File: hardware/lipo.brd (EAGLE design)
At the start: 33.5 x 34.6 mm, 57 parts, among them J1 MICRO_USB_B_HIROSE_ZX62-B-5PA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, Q1 IRLML6402, SW1 TVAF06-A020B-R, U1 LT6106CS5#PBF, U2 NJM12888F, U3 MCP73831, U5 TCK106AF,LF, X1 FA-238

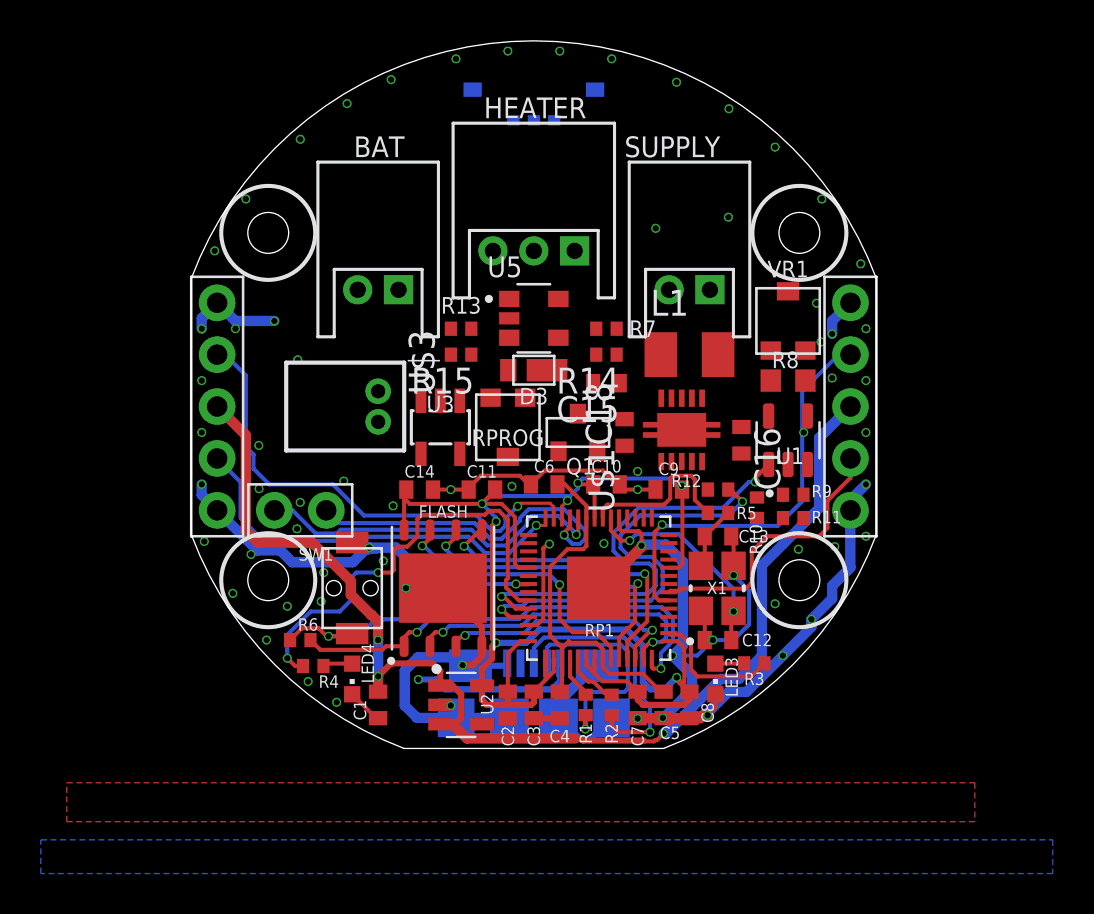
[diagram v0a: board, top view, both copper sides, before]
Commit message: アナログ入力を修正
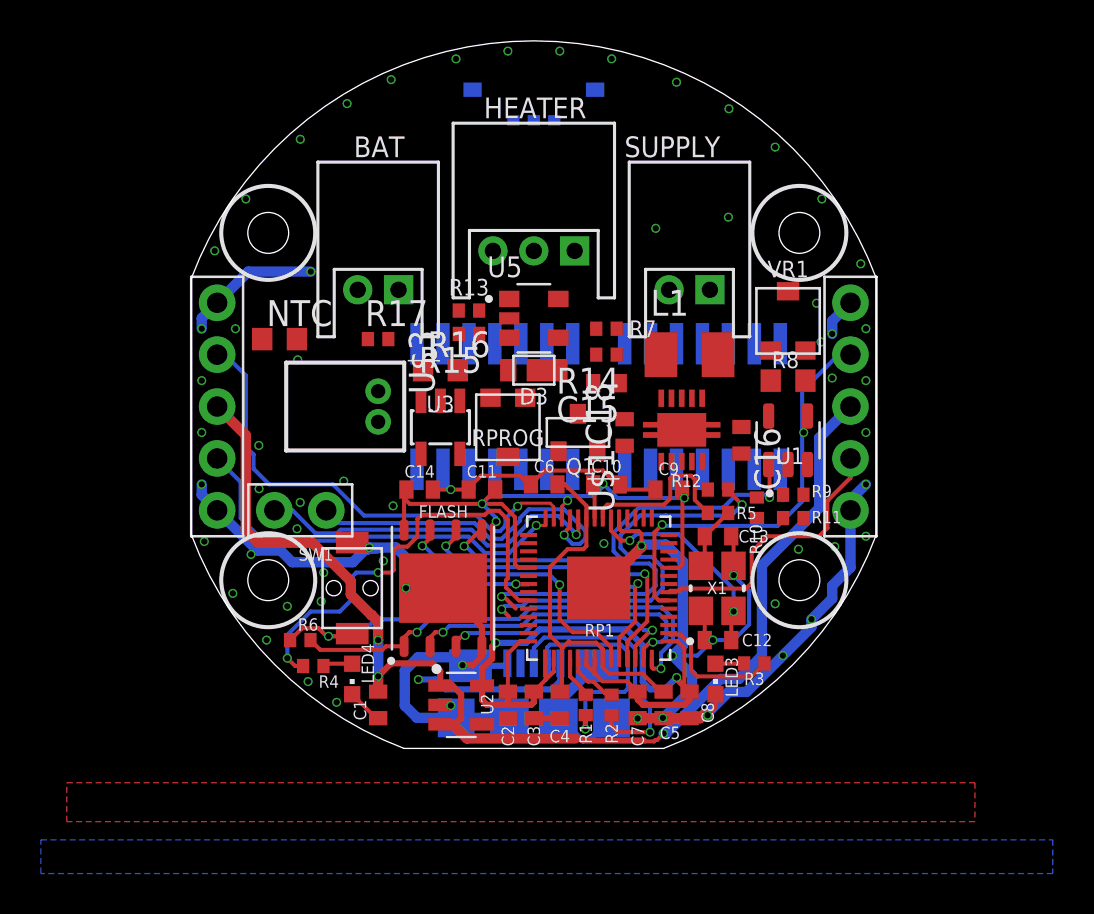
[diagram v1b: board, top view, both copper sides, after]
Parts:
- added IC1, IC2: 4066D, 40xx:SO14
- added NTC: 10k, rcl:R0603
- added R16: 0.033, rcl:R0603
- added R17: 10k, rcl:R0402
- moved R15 1.09 mm to (-3.17, 3.56)
- moved R13 0.97 mm to (-3.17, 4.70)
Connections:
- removed net ADC3: RP1.41
- removed net I2C0_SDA: RP1.11
- removed net I2C1_SCL: RP1.9
- removed net I2C1_SDA: RP1.8
- removed net I2C_SCL: RP1.12
- removed net PWM0_B: RP1.3
- removed net PWM1_A: RP1.4
- removed net PWM1_B: RP1.5
- removed net PWM3_A: RP1.34
- removed net PWM4_A: RP1.36
- removed net PWM5_A: RP1.13
- removed net PWM5_B: RP1.14
- removed net SPI0_CS: RP1.32
- removed net SPI0_MISO: RP1.31
- removed net SPI0_MOSI: RP1.30
- removed net SPI0_SCK: RP1.29
- removed net SPI1_CS: RP1.16
- removed net SPI1_MISO: RP1.15
- removed net SPI1_MOSI: RP1.18
- removed net SPI1_SCK: RP1.17
- new net ADC0_IN: IC1.2, IC1.3, RP1.38
- new net ADC1_IN: IC1.10, IC1.9, RP1.39
- new net ADC2_IN: IC2.2, IC2.3, IC2.9, RP1.40
- new net ADC_SEL1: IC1.13, IC1.6, IC2.13
- new net ADC_SEL2: IC1.12, IC1.5, IC2.5
- new net ADC_SEL3: IC2.6
- new net HEATER_I: HEATER.2, IC1.11, R16.2
- new net OB_TEMP: IC2.8, NTC.2, R17.1
- new net VSS: IC1.7, IC2.7
- net BAT_V: now also IC1.4; no longer RP1.39
- net GND: now also NTC.1, R16.1; no longer HEATER.2
- net SUPPLY_V: now also IC1.1
- net TEMP: now also IC2.4; no longer RP1.40
- net V+_I: now also IC1.8; no longer RP1.38
- net V+_V: now also IC2.1
- net VDD: now also IC1.14, IC2.14, R17.2
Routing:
- net TEMP: track 4.68 -> 0.00 mm, vias 1 -> 0
- net GND: track 117.5 -> 119.6 mm, vias 67 -> 64
- net BAT_V: track 21.5 -> 20.5 mm
